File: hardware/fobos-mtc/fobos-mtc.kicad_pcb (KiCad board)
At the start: 2 copper layers, 76.2 x 40.6 mm, 52 parts, among them J1 Conn_01x10, J10 Conn_02x10_Odd_Even, J11 Conn_02x10_Odd_Even, J12 Conn_02x06_Top_Bottom, J13 Conn_02x06_Top_Bottom, J2 Conn_01x10, J3 Conn_01x10, J4 Conn_01x10, J5 Target, J6 Conn_01x02, J7 clk, J8 Glitch, J9 Measure, Q1 BSS138, Q2 BSS84, U1 SP3003-04ATG, U2 SP3003-04ATG, U3 SP3003-04ATG

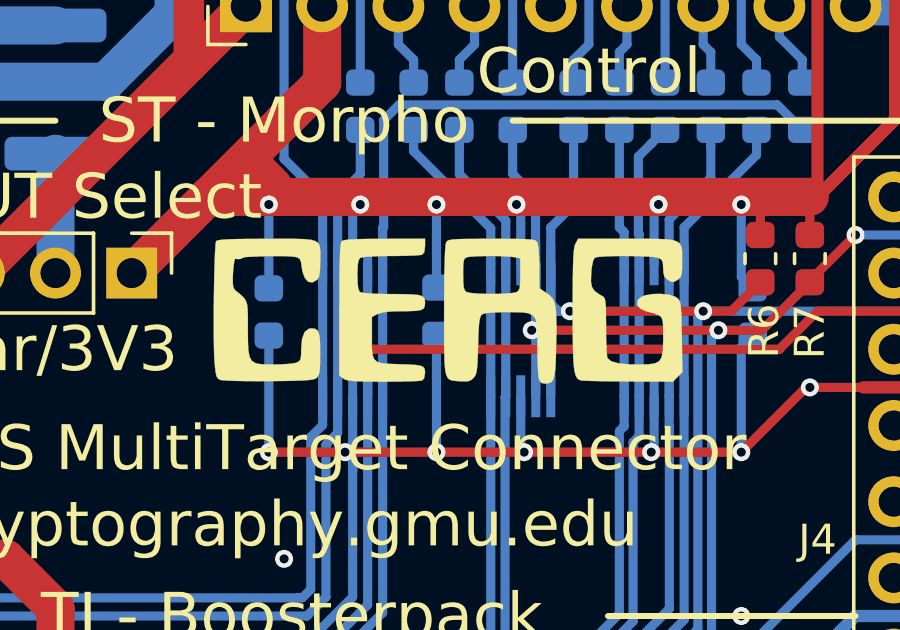
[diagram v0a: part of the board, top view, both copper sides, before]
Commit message: more pcb library cleanup
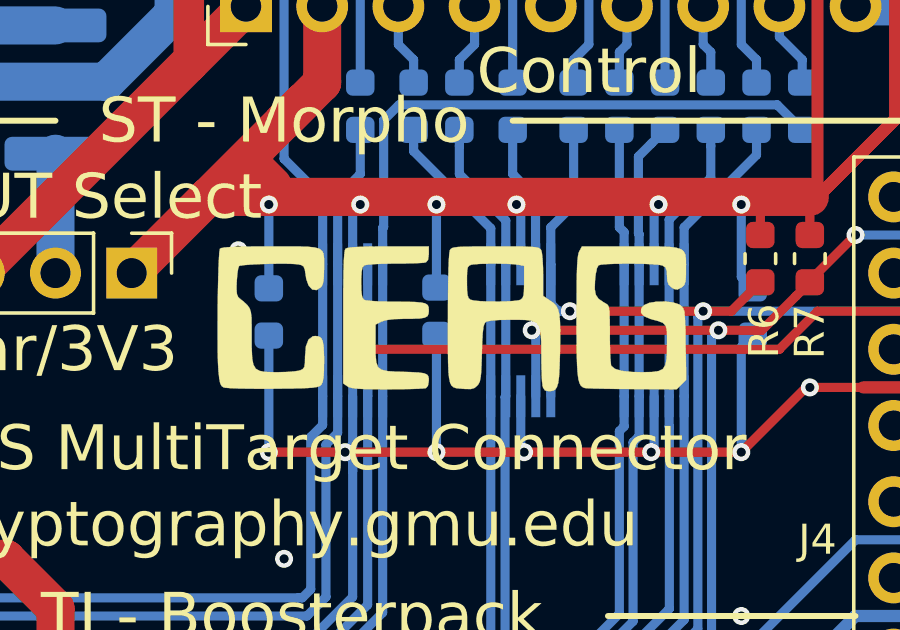
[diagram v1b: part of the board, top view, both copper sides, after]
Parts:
- removed the G*** at (140.1, 82.5)
- added G***: LOGO, cerg:cerg_logo, F.Cu at (140.2, 82.8)
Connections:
- U1 pad 10: RST -> (no net)
- U1 pad 6: DIO1 -> (no net)
- U1 pad 7: DIO0 -> (no net)
- U1 pad 9: IO -> (no net)
- U2 pad 10: Ready -> (no net)
- U2 pad 6: DIO3 -> (no net)
- U2 pad 7: Valid -> (no net)
- U2 pad 9: DIO2 -> (no net)
- U3 pad 10: CLK_D2C -> (no net)
- U3 pad 6: Aux -> (no net)
- U3 pad 7: TFD -> (no net)
- U3 pad 9: CLK_C2D -> (no net)
